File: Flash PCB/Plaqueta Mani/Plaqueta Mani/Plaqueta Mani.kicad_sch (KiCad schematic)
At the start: 1 part, among them J1 Arduino_Nano_Header

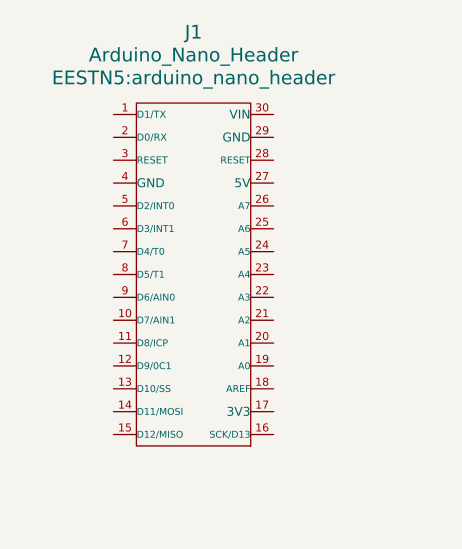
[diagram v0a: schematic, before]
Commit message: Arreglando errores de diseño
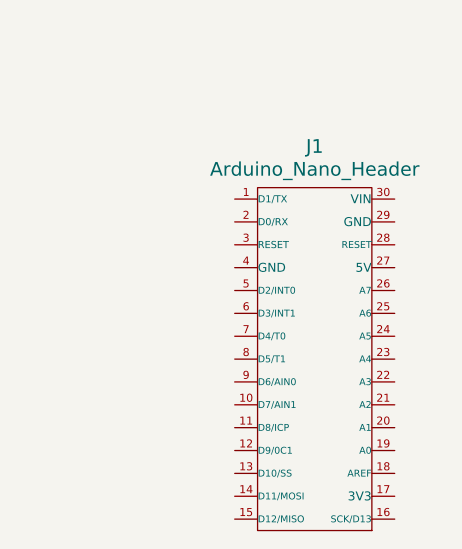
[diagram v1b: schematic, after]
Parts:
- J1: footprint EESTN5:arduino_nano_header -> (none)
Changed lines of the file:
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@@
 (kicad_sch (version 20230121) (generator eeschema)
   (paper "A4")
-  (symbol (lib_id "EESTN5:Arduino_Nano_Header") (at 132.334 72.644 0) (unit 1)
+  (symbol (lib_id "EESTN5:Arduino_Nano_Header") (at 145.796 82.042 0) (unit 1)
     (in_bom yes) (on_board yes) (dnp no) (fields_autoplaced)
-    (property "Reference" "J1" (at 132.334 45.72 0)
+    (property "Reference" "J1" (at 145.796 58.42 0)
       (effects (font (size 1.524 1.524)))
     )
-    (property "Value" "Arduino_Nano_Header" (at 132.334 48.26 0)
+    (property "Value" "Arduino_Nano_Header" (at 145.796 60.96 0)
       (effects (font (size 1.524 1.524)))
     )
-    (property "Footprint" "EESTN5:arduino_nano_header" (at 132.334 50.8 0)
+    (property "Footprint" "" (at 145.796 82.042 0)
       (effects (font (size 1.524 1.524)))
     )
-    (property "Datasheet" "" (at 132.334 72.644 0)
+    (property "Datasheet" "" (at 145.796 82.042 0)
       (effects (font (size 1.524 1.524)))
     )
@@
     (pin "9")
     (instances
-      (project "Flash Forma"
-        (path "/17d5f0a9-f2e8-4c5a-bea9-93a856536820"
+      (project "Plaqueta Mani"
+        (path "/b1c9236c-08e5-42c5-bca3-c7d41737a702"
           (reference "J1") (unit 1)
         )
